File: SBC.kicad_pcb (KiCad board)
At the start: 2 copper layers, 160 x 100.3 mm, 93 parts, among them K1 CONN_3, K10 CONN_3, K11 CONN_3, K12 CONN_3, K13 CONN_3, K2 CONN_3, K3 CONN_3, K4 CONN_3, K5 CONN_3, K6 CONN_3, K7 CONN_3, K8 CONN_3, K9 CONN_3, P1 PARALLEL, P2 POWER, P3 SERIAL, P4 CLK_CPU, P5 CLK_UART, P6 RESET, SW1 SW_PUSH, U1 16550, U10 74LS243, U11 74LS245, U12 74LS174, U13 74LS174, U14 74LS32, U15 74LS32, U16 74LS32, U17 74LS244, U18 74LS174, U19 8255, U2 27C080, U20 C96ABC, U21 DS1302, U22 MAX232, U23 SRAM_512KO, U24 Z80-CPU, U25 DS1210, U26 74LS06N, U3 74LS08, U4 74LS10, U5 74LS125, U6 74LS139, U7 74LS14, U8 74LS245, U9 74LS245, X1 CRYSTAL

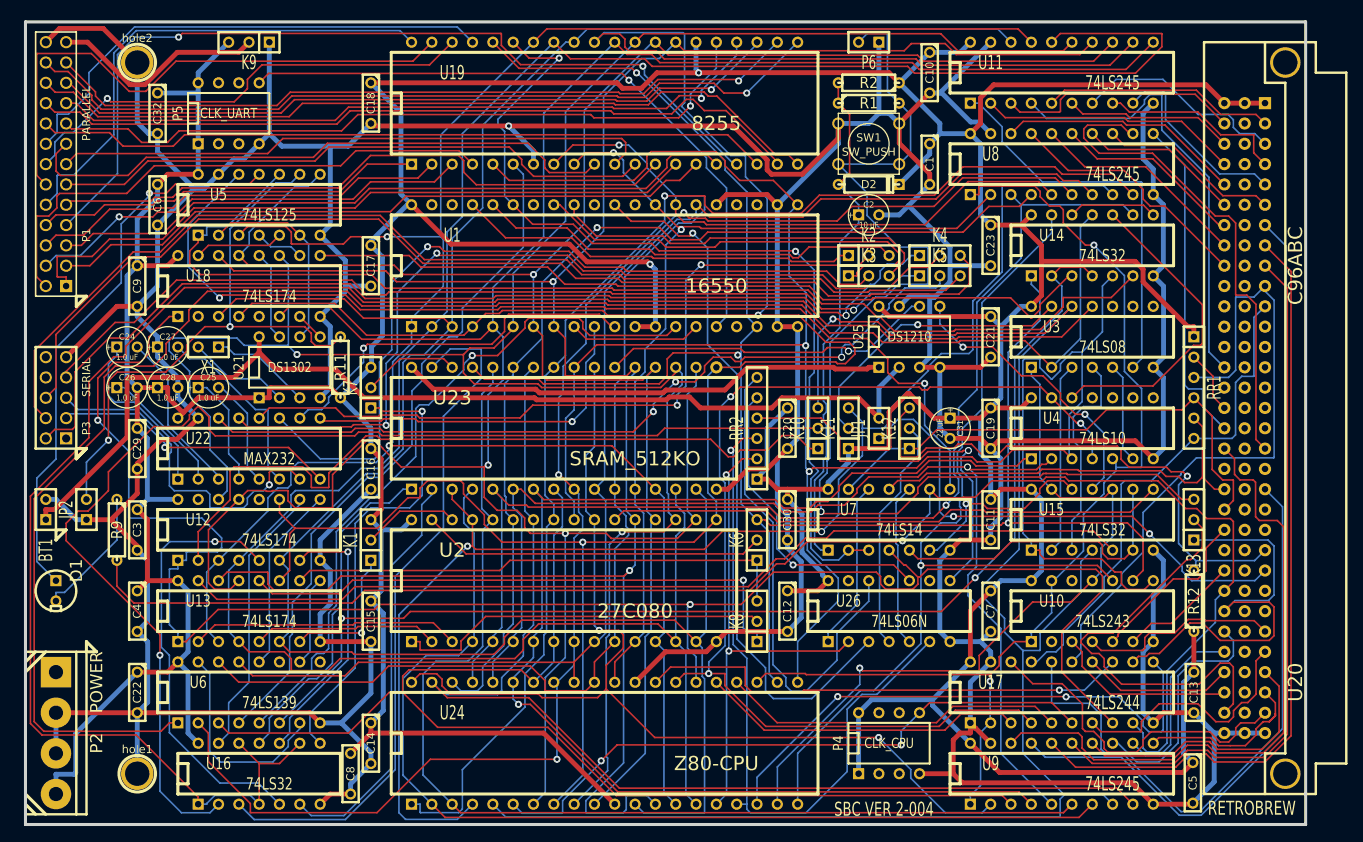
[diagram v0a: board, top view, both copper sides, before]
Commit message: Version B
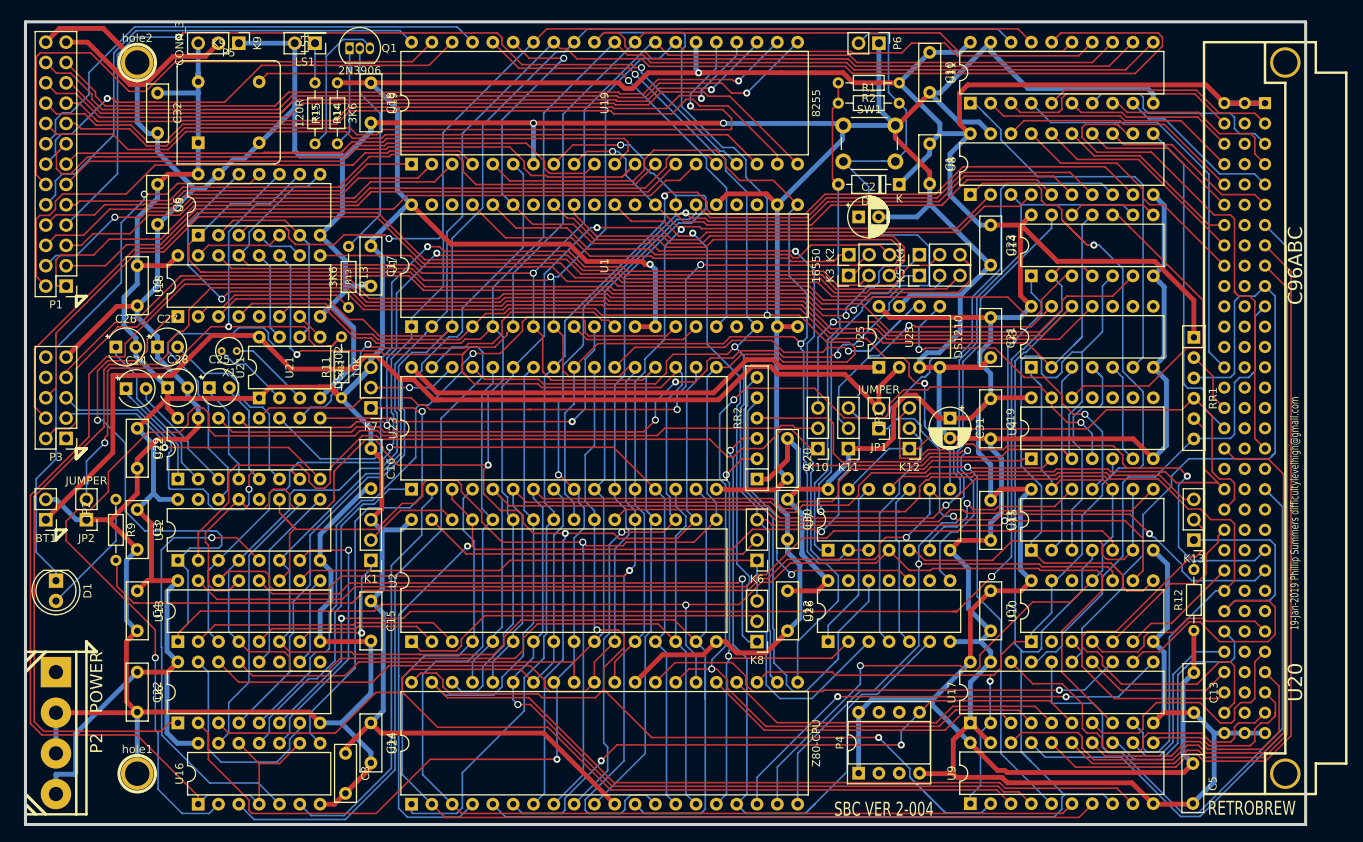
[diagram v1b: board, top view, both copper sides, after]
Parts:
- added LS1: Speaker, Connector_PinHeader_2.54mm:PinHeader_2x01_P2.54mm_Vertical, F.Cu at (113.7, 56.0)
- added Q1: 2N3906, Package_TO_SOT_THT:TO-92_Inline, F.Cu at (118.0, 56.6)
- added R13: 3K6, Resistor_THT:R_Axial_DIN0204_L3.6mm_D1.6mm_P7.62mm_Horizontal, F.Cu at (117.9, 81.4)
- added R14: 3K6, Resistor_THT:R_Axial_DIN0204_L3.6mm_D1.6mm_P7.62mm_Horizontal, F.Cu at (116.5, 68.6)
- added R15: 120R, Resistor_THT:R_Axial_DIN0204_L3.6mm_D1.6mm_P7.62mm_Horizontal, F.Cu at (113.7, 61.0)
- BT1, JP1, JP2, P6: footprint SIL-2 -> Connector_PinHeader_2.54mm:PinHeader_1x02_P2.54mm_Vertical
- C1, C10, C11, C12, C13, C14, C15, C16, C17, C18, C19, C20, C21, C22, C23, C29, C3, C30, C32, C4, C5, C6, C7, C8, C9: footprint C2 -> Capacitor_THT:C_Disc_D7.0mm_W2.5mm_P5.00mm
- C2, C31: footprint C1V5 -> Capacitor_THT:CP_Radial_D5.0mm_P2.50mm
- C24, C25, C26, C27, C28: footprint C1V5 -> Capacitor_THT:CP_Radial_Tantal_D4.5mm_P2.50mm
- D1: footprint LEDV -> LED_THT:LED_D5.0mm
- D2: value DIODE -> 1N4148; footprint D3 -> Diode_THT:D_DO-35_SOD27_P7.62mm_Horizontal
- K1, K10, K11, K12, K13, K2, K3, K4, K5, K6, K7, K8, K9: footprint SIL-3 -> Connector_PinHeader_2.54mm:PinHeader_1x03_P2.54mm_Vertical
- P1: footprint pin_array_13x2 -> Connector_PinHeader_2.54mm:PinHeader_2x13_P2.54mm_Vertical
- P3: footprint PIN_ARRAY_5x2 -> Connector_PinHeader_2.54mm:PinHeader_2x05_P2.54mm_Vertical
- P4: footprint 8dip300 -> Package_DIP:DIP-8_W7.62mm_Socket
- P5: footprint 8dip300 -> Oscillator:Oscillator_DIP-8
- R1: value 10 -> 10R; footprint R3 -> Resistor_THT:R_Axial_DIN0204_L3.6mm_D1.6mm_P7.62mm_Horizontal
- R11, R12, R2, R9: footprint R3 -> Resistor_THT:R_Axial_DIN0204_L3.6mm_D1.6mm_P7.62mm_Horizontal
- RR1, RR2: footprint SIL-6 -> Resistor_THT:R_Array_SIP6
- SW1: footprint SW_PUSH_SMALL -> Button_Switch_THT:SW_PUSH_6mm_H8mm
- U1, U19, U24: footprint 40dip600 -> Package_DIP:DIP-40_W15.24mm
- U10, U14, U15, U16, U26, U3, U4, U5, U7: footprint 14dip300 -> Package_DIP:DIP-14_W7.62mm
- U11, U17, U8, U9: footprint 20dip300 -> Package_DIP:DIP-20_W7.62mm
- U12, U13, U18, U22, U6: footprint 16dip300 -> Package_DIP:DIP-16_W7.62mm
- U2, U23: footprint 32dip600 -> Package_DIP:DIP-32_W15.24mm
- U21, U25: footprint 8dip300 -> Package_DIP:DIP-8_W7.62mm
- X1: footprint SIL-2 -> Crystal:Crystal_Round_D3.0mm_Vertical
- moved U1 25.3 mm to (125.7, 91.4), turned to 90 degrees
- moved U19 25.3 mm to (125.7, 71.1), turned to 90 degrees
- moved U24 25.3 mm to (125.7, 151.1), turned to 90 degrees
- moved U2 20.5 mm to (125.7, 130.8), turned to 90 degrees
- moved U23 20.5 mm to (125.7, 111.8), turned to 90 degrees
- moved P1 15.3 mm to (82.5, 86.4), turned to 180 degrees
- moved U11 12.0 mm to (195.6, 63.5), turned to 90 degrees
- moved U17 12.0 mm to (195.6, 141.0), turned to 90 degrees
- moved U8 12.0 mm to (195.6, 74.9), turned to 90 degrees
- moved U9 12.0 mm to (195.6, 151.1), turned to 90 degrees
- moved U12 9.67 mm to (96.5, 120.7), turned to 90 degrees
- moved U13 9.67 mm to (96.5, 130.8), turned to 90 degrees
- moved U18 9.67 mm to (96.5, 90.2), turned to 90 degrees
- moved U6 9.67 mm to (96.5, 141.0), turned to 90 degrees
- moved U22 9.67 mm to (96.5, 110.5), turned to 90 degrees
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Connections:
- D2 pad 1: Net-(C2-Pad1) -> VCC
- D2 pad 2: VCC -> Net-(C2-Pad1)
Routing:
- net GND: track 833.8 -> 881.5 mm, vias 1 -> 2
- net VCC: track 788.3 -> 829.7 mm
- net Net-(Q1-Pad2): track 0.00 -> 27.5 mm
- net Net-(R13-Pad2): track 0.00 -> 20.5 mm
- net Net-(Q1-Pad3): track 0.00 -> 18.4 mm
- net Net-(Q1-Pad1): track 0.00 -> 13.1 mm
- net /PB7: track 90.6 -> 102.3 mm
- net /PC6: track 74.7 -> 85.7 mm
- net //HALT: track 69.6 -> 58.9 mm
- net Net-(U23-Pad22): track 42.0 -> 52.7 mm
- net Net-(C24-Pad1): track 22.0 -> 14.7 mm
- net //RD: track 274.0 -> 281.2 mm
- net //BUSAK: track 136.3 -> 143.5 mm
- net /A10: track 127.4 -> 134.4 mm
- net /D4: track 307.0 -> 313.6 mm
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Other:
- board text added: "19-Jan-2019 Phillip Summers difficultylevelhigh@gmail.com"

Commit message: Version C
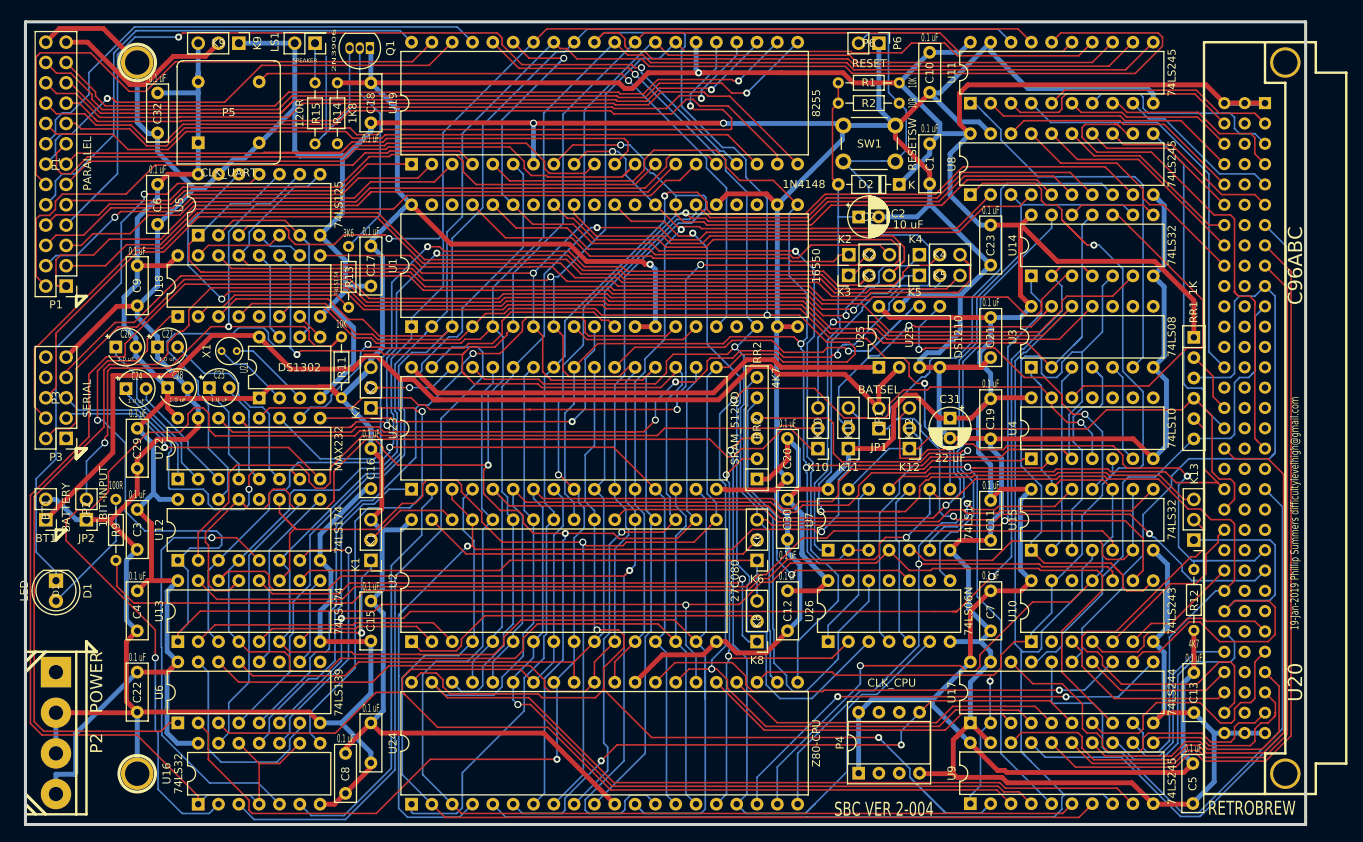
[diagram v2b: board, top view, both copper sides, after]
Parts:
- JP1: value JUMPER -> BATSEL
- JP2: value JUMPER -> 1BIT-INPUT
- LS1: value Speaker -> SPEAKER
- R12, RR2: value 4700 -> 4K7
- R14: value 3K6 -> 1K8
- R9: value 100 -> 100R
- RR1: value 1000 -> 1K
- SW1: value SW_PUSH -> RESETSW
- moved Q1 2.54 mm to (120.5, 56.6), turned to 180 degrees
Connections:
- Q1 pad 1: Net-(Q1-Pad1) -> VCC
- R14 pad 1: Net-(Q1-Pad1) -> Net-(R14-Pad1)
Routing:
- net Net-(Q1-Pad1): track 13.1 -> 0.00 mm
- net Net-(Q1-Pad3): track 18.4 -> 23.8 mm
- net VCC: track 829.7 -> 834.3 mm
- net Net-(C2-Pad1): track 61.7 -> 64.2 mm
